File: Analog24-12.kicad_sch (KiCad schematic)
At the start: 15 parts, among them J1 Conn_01x02

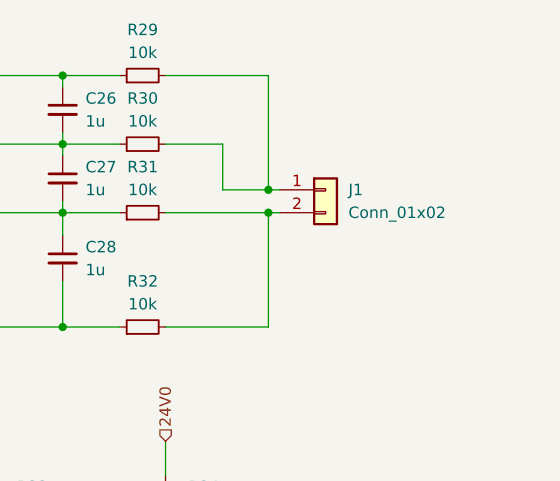
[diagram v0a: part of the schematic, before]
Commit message: place
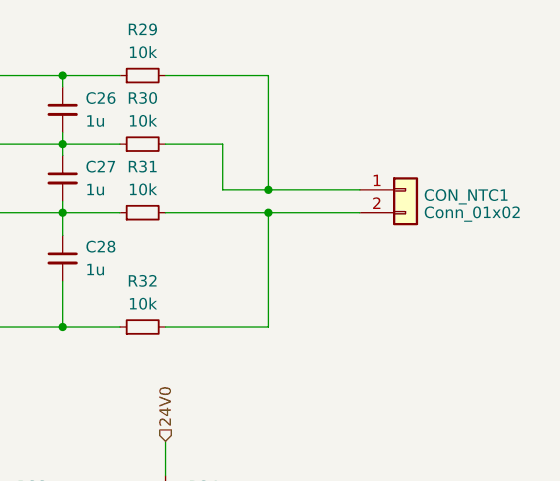
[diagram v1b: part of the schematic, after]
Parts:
- C26, C27, C28, C29, C30: footprint (none) -> Capacitor_SMD:C_0603_1608Metric_Pad1.08x0.95mm_HandSolder
- CON_NTC1: renamed from J1; footprint (none) -> Connector_Phoenix_MSTB:PhoenixContact_MSTBA_2,5_2-G-5,08_1x02_P5.08mm_Horizontal
- R29, R30, R31, R32, R33, R34, R35, R36: footprint (none) -> Resistor_SMD:R_0805_2012Metric_Pad1.20x1.40mm_HandSolder
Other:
- moved on the sheet: CON_NTC1
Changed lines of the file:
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@@
     (stroke (width 0) (type default))
   )
-  (wire (pts (xy 241.3 53.34) (xy 242.57 53.34))
+  (wire (pts (xy 241.3 53.34) (xy 251.46 53.34))
     (stroke (width 0) (type default))
   )
@@
     (stroke (width 0) (type default))
   )
-  (wire (pts (xy 241.3 55.88) (xy 242.57 55.88))
+  (wire (pts (xy 241.3 55.88) (xy 251.46 55.88))
     (stroke (width 0) (type default))
   )
@@
       (effects (font (size 1.27 1.27)))
     )
-    (property "Footprint" "" (at 227.33 55.88 0)
+    (property "Footprint" "Resistor_SMD:R_0805_2012Metric_Pad1.20x1.40mm_HandSolder" (at 227.33 55.88 0)
       (effects (font (size 1.27 1.27)) hide)
     )
@@
       (effects (font (size 1.27 1.27)) (justify left))
     )
-    (property "Footprint" "" (at 229.87 96.52 0)
+    (property "Footprint" "Resistor_SMD:R_0805_2012Metric_Pad1.20x1.40mm_HandSolder" (at 229.87 96.52 0)
       (effects (font (size 1.27 1.27)) hide)
     )
@@
       (effects (font (size 1.27 1.27)) (justify left))
     )
-    (property "Footprint" "" (at 229.87 87.63 0)
+    (property "Footprint" "Resistor_SMD:R_0805_2012Metric_Pad1.20x1.40mm_HandSolder" (at 229.87 87.63 0)
       (effects (font (size 1.27 1.27)) hide)
     )
@@
       (effects (font (size 1.27 1.27)) (justify left))
     )
-    (property "Footprint" "" (at 218.44 52.07 0)
+    (property "Footprint" "Capacitor_SMD:C_0603_1608Metric_Pad1.08x0.95mm_HandSolder" (at 218.44 52.07 0)
       (effects (font (size 1.27 1.27)) hide)
     )
@@
       (effects (font (size 1.27 1.27)))
     )
-    (property "Footprint" "" (at 227.33 48.26 0)
+    (property "Footprint" "Resistor_SMD:R_0805_2012Metric_Pad1.20x1.40mm_HandSolder" (at 227.33 48.26 0)
       (effects (font (size 1.27 1.27)) hide)
     )
@@
       (effects (font (size 1.27 1.27)) (justify left))
     )
-    (property "Footprint" "" (at 218.44 60.96 0)
+    (property "Footprint" "Capacitor_SMD:C_0603_1608Metric_Pad1.08x0.95mm_HandSolder" (at 218.44 60.96 0)
       (effects (font (size 1.27 1.27)) hide)
     )
@@
       (effects (font (size 1.27 1.27)))
     )
-    (property "Footprint" "" (at 227.33 40.64 0)
+    (property "Footprint" "Resistor_SMD:R_0805_2012Metric_Pad1.20x1.40mm_HandSolder" (at 227.33 40.64 0)
       (effects (font (size 1.27 1.27)) hide)
     )
@@
       (effects (font (size 1.27 1.27)) (justify left))
     )
-    (property "Footprint" "" (at 218.44 44.45 0)
+    (property "Footprint" "Capacitor_SMD:C_0603_1608Metric_Pad1.08x0.95mm_HandSolder" (at 218.44 44.45 0)
       (effects (font (size 1.27 1.27)) hide)
     )
@@
       (effects (font (size 1.27 1.27)) (justify left))
     )
-    (property "Footprint" "" (at 210.82 87.63 0)
+    (property "Footprint" "Resistor_SMD:R_0805_2012Metric_Pad1.20x1.40mm_HandSolder" (at 210.82 87.63 0)
       (effects (font (size 1.27 1.27)) hide)
     )
@@
       (effects (font (size 1.27 1.27)) (justify left))
     )
-    (property "Footprint" "" (at 210.82 96.52 0)
+    (property "Footprint" "Resistor_SMD:R_0805_2012Metric_Pad1.20x1.40mm_HandSolder" (at 210.82 96.52 0)
       (effects (font (size 1.27 1.27)) hide)
     )
@@
     )
   )
-  (symbol (lib_id "Connector_Generic:Conn_01x02") (at 247.65 53.34 0) (unit 1)
-    (in_bom yes) (on_board yes) (dnp no) (fields_autoplaced)
-    (property "Reference" "J1" (at 250.19 53.34 0)
-      (effects (font (size 1.27 1.27)) (justify left))
-    )
-    (property "Value" "Conn_01x02" (at 250.19 55.88 0)
-      (effects (font (size 1.27 1.27)) (justify left))
-    )
-    (property "Footprint" "" (at 247.65 53.34 0)
-      (effects (font (size 1.27 1.27)) hide)
-    )
-    (property "Datasheet" "~" (at 247.65 53.34 0)
-      (effects (font (size 1.27 1.27)) hide)
-    )
-    (pin "1")
-    (pin "2")
-    (instances
-      (project "rollo control"
-        (path "/7fd4875b-e2b3-49e9-a377-320ee6c6aef7/4430fecd-b2bb-44df-a0b9-accae9d9e5ff"
-          (reference "J1") (unit 1)
+  (symbol (lib_id "Connector_Generic:Conn_01x02") (at 256.54 53.34 0) (unit 1)
+    (in_bom yes) (on_board yes) (dnp no) (fields_autoplaced)
+    (property "Reference" "CON_NTC1" (at 258.572 53.9663 0)
+      (effects (font (size 1.27 1.27)) (justify left))
+    )
+    (property "Value" "Conn_01x02" (at 258.572 55.8873 0)
+      (effects (font (size 1.27 1.27)) (justify left))
+    )
+    (property "Footprint" "Connector_Phoenix_MSTB:PhoenixContact_MSTBA_2,5_2-G-5,08_1x02_P5.08mm_Horizontal" (at 256.54 53.34 0)
+      (effects (font (size 1.27 1.27)) hide)
+    )
+    (property "Datasheet" "~" (at 256.54 53.34 0)
+      (effects (font (size 1.27 1.27)) hide)
+    )
+    (pin "1")
+    (pin "2")
+    (instances
+      (project "rollo control"
+        (path "/7fd4875b-e2b3-49e9-a377-320ee6c6aef7/4430fecd-b2bb-44df-a0b9-accae9d9e5ff"
+          (reference "CON_NTC1") (unit 1)
         )
       )
@@
       (effects (font (size 1.27 1.27)) (justify left))
     )
-    (property "Footprint" "" (at 198.12 97.79 0)
+    (property "Footprint" "Capacitor_SMD:C_0603_1608Metric_Pad1.08x0.95mm_HandSolder" (at 198.12 97.79 0)
       (effects (font (size 1.27 1.27)) hide)
     )
@@
       (effects (font (size 1.27 1.27)))
     )
-    (property "Footprint" "" (at 227.33 68.58 0)
+    (property "Footprint" "Resistor_SMD:R_0805_2012Metric_Pad1.20x1.40mm_HandSolder" (at 227.33 68.58 0)
       (effects (font (size 1.27 1.27)) hide)
     )
@@
       (effects (font (size 1.27 1.27)) (justify left))
     )
-    (property "Footprint" "" (at 242.57 97.79 0)
-      (effects (font (size 1.27 1.27)) hide)
-    )
+    (property "Footprint" "Capacitor_SMD:C_0603_1608Metric_Pad1.08x0.95mm_HandSolder" (at 242.57 97.79 0)
+      (effects (font (size 1.27 1.27)) hide)
+    )
